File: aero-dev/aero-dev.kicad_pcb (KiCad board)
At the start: 2 copper layers, 58 x 58 mm, 58 parts, among them J1 Conn_01x03_Pin, J2 USB_C_Receptacle_USB2.0_16P, J3 Conn_ARM_SWD_TagConnect_TC203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, J4 Conn_01x03_Pin, J5 Conn_01x03_Pin, J6 Conn_01x03_Pin, J7 Barrel_Jack_Switch, U1 TPS5450DDAR, U2 TPS5450DDAR, U4 SRV05-4, U5 STM32F103C8Tx, U6 AMS1117-3.3, Y1 16MHz

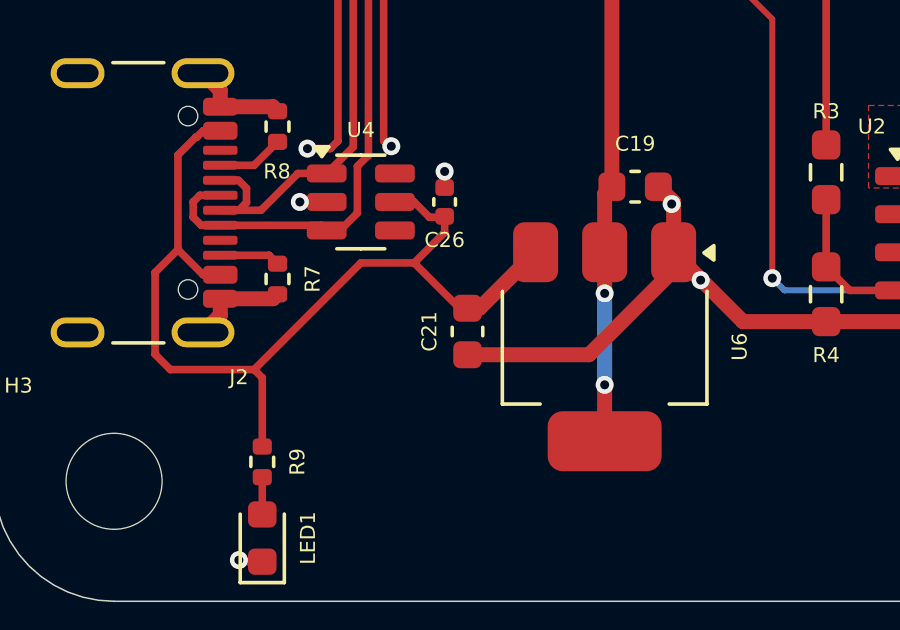
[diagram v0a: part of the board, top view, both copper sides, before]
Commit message: Finalize production files and minor edits
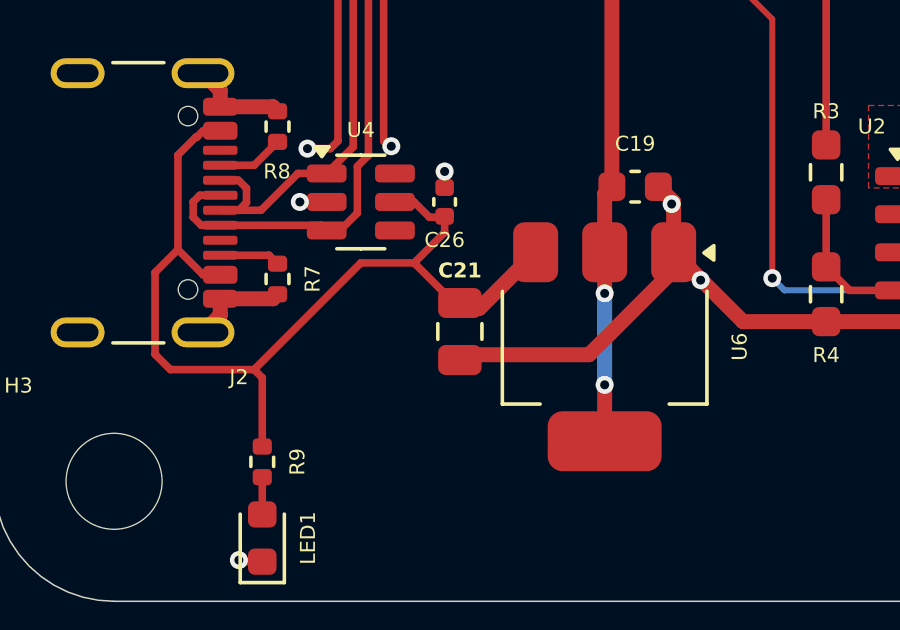
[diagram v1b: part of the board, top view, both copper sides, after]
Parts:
- C21: footprint Capacitor_SMD:C_0603_1608Metric -> Capacitor_SMD:C_0805_2012Metric
- moved C21 0.25 mm to (71.6, 81.5)
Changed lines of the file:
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@@
 		(sheetname "Root")
 		(sheetfile "aero-dev.kicad_sch")
-		(attr through_hole)
+		(attr through_hole dnp)
 		(fp_line
 			(start -1.33 -1.33)
@@
 			)
 		)
+		(property "LCSC" "C2986058"
+			(at 0 0 0)
+			(unlocked yes)
+			(layer "F.Fab")
+			(hide yes)
+			(effects
+				(font
+					(size 1 1)
+					(thickness 0.15)
+				)
+			)
+		)
 		(property ki_fp_filters "LED* LED_SMD:* LED_THT:*")
 		(sheetname "Regulator2")
@@
 		(sheetname "Root")
 		(sheetfile "aero-dev.kicad_sch")
-		(attr through_hole)
+		(attr through_hole dnp)
 		(fp_line
 			(start -1.33 6.409999)
@@
 		)
 	)
-	(footprint "Capacitor_SMD:C_0603_1608Metric"
+	(footprint "Capacitor_SMD:C_0805_2012Metric"
 		(layer "F.Cu")
-		(at 71.882 81.534 -90)
-		(descr "Capacitor SMD 0603 (1608 Metric), square (rectangular) end terminal, IPC_7351 nominal, (Body size source: IPC-SM-782 page 76, https://www.pcb-3d.com/wordpress/wp-content/uploads/ipc-sm-782a_amendment_1_and_2.pdf), generated with kicad-footprint-generator")
+		(at 71.628 81.534 -90)
+		(descr "Capacitor SMD 0805 (2012 Metric), square (rectangular) end terminal, IPC_7351 nominal, (Body size source: IPC-SM-782 page 76, https://www.pcb-3d.com/wordpress/wp-content/uploads/ipc-sm-782a_amendment_1_and_2.pdf, https://docs.google.com/spreadsheets/d/1BsfQQcO9C6DZCsRaXUlFlo91Tg2WpOkGARC1WS5S8t0/edit?usp=sharing), generated with kicad-footprint-generator")
 		(tags "capacitor")
 		(property "Reference" "C21"
-			(at 0 1.27 90)
+			(at -2.032 0 0)
 			(layer "F.SilkS")
 			(effects
@@
 					(size 0.5 0.5)
 					(thickness 0.1)
+					(bold yes)
 				)
 			)
 		)
 		(property "Value" "22u"
-			(at 0 1.43 90)
+			(at 0 1.68 -90)
 			(layer "F.Fab")
 			(effects
@@
 			)
 		)
-		(property "Footprint" "Capacitor_SMD:C_0603_1608Metric"
+		(property "Footprint" "Capacitor_SMD:C_0805_2012Metric"
 			(at 0 0 -90)
 			(unlocked yes)
@@
 		(attr smd)
 		(fp_line
-			(start -0.140581 0.51)
-			(end 0.140581 0.51)
+			(start -0.261252 0.735)
+			(end 0.261252 0.735)
 			(stroke
 				(width 0.12)
@@
 		)
 		(fp_line
-			(start -0.140581 -0.51)
-			(end 0.140581 -0.51)
+			(start -0.261252 -0.735)
+			(end 0.261252 -0.735)
 			(stroke
 				(width 0.12)
@@
 		)
 		(fp_line
-			(start -1.48 0.73)
-			(end -1.48 -0.73)
+			(start -1.7 0.98)
+			(end -1.7 -0.98)
 			(stroke
 				(width 0.05)
@@
 		)
 		(fp_line
-			(start 1.48 0.73)
-			(end -1.48 0.73)
+			(start 1.7 0.98)
+			(end -1.7 0.98)
 			(stroke
 				(width 0.05)
@@
 		)
 		(fp_line
-			(start -1.48 -0.73)
-			(end 1.48 -0.73)
+			(start -1.7 -0.98)
+			(end 1.7 -0.98)
 			(stroke
 				(width 0.05)
@@
 		)
 		(fp_line
-			(start 1.48 -0.73)
-			(end 1.48 0.73)
+			(start 1.7 -0.98)
+			(end 1.7 0.98)
 			(stroke
 				(width 0.05)
@@
 		)
 		(fp_line
-			(start -0.8 0.4)
-			(end -0.8 -0.4)
+			(start -1 0.625)
+			(end -1 -0.625)
 			(stroke
 				(width 0.1)
@@
 		)
 		(fp_line
-			(start 0.8 0.4)
-			(end -0.8 0.4)
+			(start 1 0.625)
+			(end -1 0.625)
 			(stroke
 				(width 0.1)
@@
 		)
 		(fp_line
-			(start -0.8 -0.4)
-			(end 0.8 -0.4)
+			(start -1 -0.625)
+			(end 1 -0.625)
 			(stroke
 				(width 0.1)
@@
 		)
 		(fp_line
-			(start 0.8 -0.4)
-			(end 0.8 0.4)
+			(start 1 -0.625)
+			(end 1 0.625)
 			(stroke
 				(width 0.1)
@@
 		)
 		(fp_text user "${REFERENCE}"
-			(at 0 0 90)
+			(at 0 0 -90)
 			(layer "F.Fab")
 			(effects
 				(font
-					(size 0.4 0.4)
-					(thickness 0.06)
+					(size 0.5 0.5)
+					(thickness 0.08)
 				)
 			)
 		)
 		(pad "1" smd roundrect
-			(at -0.775 0 270)
-			(size 0.9 0.95)
+			(at -0.95 0 270)
+			(size 1 1.45)
 			(layers "F.Cu" "F.Paste" "F.Mask")
 			(roundrect_rratio 0.25)
@@
 		)
 		(pad "2" smd roundrect
-			(at 0.775 0 270)
-			(size 0.9 0.95)
+			(at 0.95 0 270)
+			(size 1 1.45)
 			(layers "F.Cu" "F.Paste" "F.Mask")
 			(roundrect_rratio 0.25)
@@
 			(pintype "passive")
 		)
-		(model "${KICAD8_3DMODEL_DIR}/Capacitor_SMD.3dshapes/C_0603_1608Metric.wrl"
+		(model "${KICAD8_3DMODEL_DIR}/Capacitor_SMD.3dshapes/C_0805_2012Metric.wrl"
 			(offset
 				(xyz 0 0 0)
@@
 			)
 		)
+		(property "LCSC" "C2986059"
+			(at 0 0 90)
+			(unlocked yes)
+			(layer "F.Fab")
+			(hide yes)
+			(effects
+				(font
+					(size 1 1)
+					(thickness 0.15)
+				)
+			)
+		)
 		(property ki_fp_filters "LED* LED_SMD:* LED_THT:*")
 		(sheetname "Root")
@@
 			)
 		)
+		(property "LCSC" "C114425"
+			(at 0 0 0)
+			(unlocked yes)
+			(layer "F.Fab")
+			(hide yes)
+			(effects
+				(font
+					(size 1 1)
+					(thickness 0.15)
+				)
+			)
+		)
 		(sheetname "Regulator1")
 		(sheetfile "regulator.kicad_sch")
@@
 			)
 		)
+		(property "LCSC" "C2986058"
+			(at 0 0 0)
+			(unlocked yes)
+			(layer "F.Fab")
+			(hide yes)
+			(effects
+				(font
+					(size 1 1)
+					(thickness 0.15)
+				)
+			)
+		)
 		(property ki_fp_filters "LED* LED_SMD:* LED_THT:*")
 		(sheetname "Regulator1")
@@
 		(sheetname "Root")
 		(sheetfile "aero-dev.kicad_sch")
-		(attr through_hole)
+		(attr through_hole dnp)
 		(fp_line
 			(start -1.33 6.409999)
@@
 			)
 		)
+		(property "LCSC" "C114425"
+			(at 0 0 0)
+			(unlocked yes)
+			(layer "F.Fab")
+			(hide yes)
+			(effects
+				(font
+					(size 1 1)
+					(thickness 0.15)
+				)
+			)
+		)
 		(sheetname "Regulator2")
 		(sheetfile "regulator.kicad_sch")
@@
 		(sheetname "Root")
 		(sheetfile "aero-dev.kicad_sch")
-		(attr through_hole)
+		(attr through_hole dnp)
 		(fp_line
 			(start -1.33 -1.33)
